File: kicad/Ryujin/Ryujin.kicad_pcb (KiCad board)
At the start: 2 copper layers, 173 x 72 mm, 61 parts, among them J1 Conn_01x02_Socket, J10 Conn_01x04_Pin, J11 Conn_01x04_Pin, J12 Conn_01x04_Pin, J2 1822972, J3 Conn_01x14_Socket, J4 Conn_01x14_Socket, J5 1822972, J6 Conn_01x04_Pin, J7 Conn_01x04_Pin, J8 Conn_01x04_Pin, J9 Conn_01x04_Pin, Q1 IRLML5203, Q2 IRLML6244, Q3 Si7288, Q4 2N7002, U1 74LVC1G17, U2 74AHCT1G14, U3 TMUX1119DBVR, U4 SHTC3, U5 W25Q32JVSS, U6 BQ24650, U7 R-78E5.0-1.0

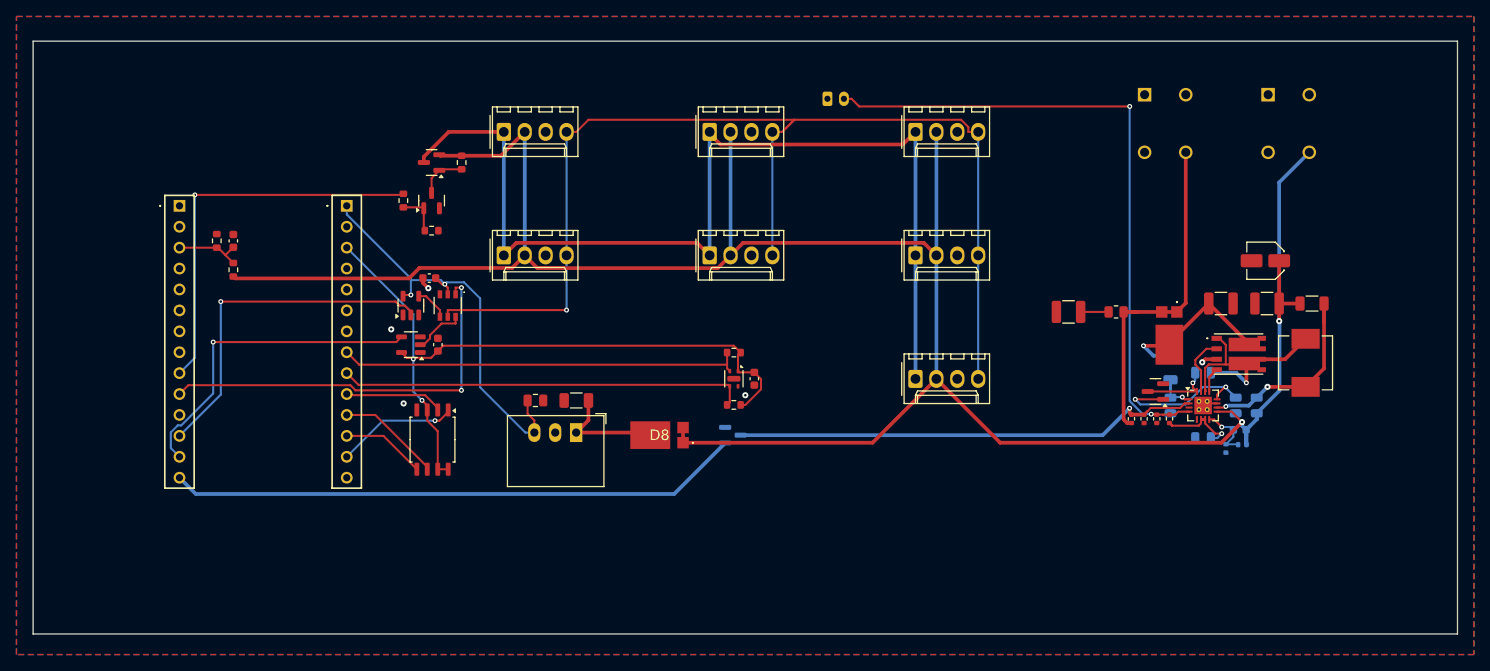
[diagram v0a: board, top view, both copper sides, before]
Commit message: In Sickness and in Hell
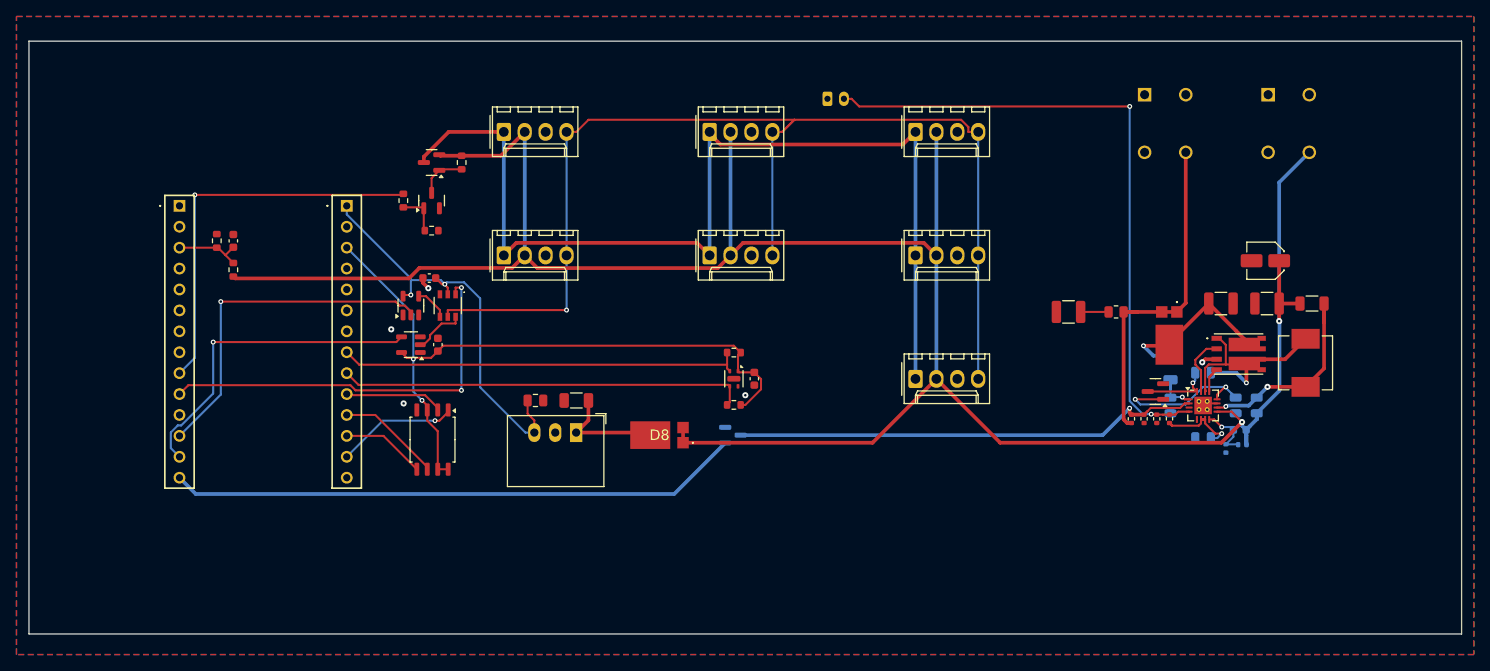
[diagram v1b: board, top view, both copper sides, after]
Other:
- board size 173 x 72 mm -> 174 x 72 mm
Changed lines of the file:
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@@
 	)
 	(gr_rect
-		(start 14.75 26.3)
-		(end 187.75 98.3)
+		(start 14.25 26.3)
+		(end 188.25 98.3)
 		(stroke
 			(width 0.05)
